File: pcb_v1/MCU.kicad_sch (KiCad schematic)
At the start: 3 parts, among them U4 ESP32-S3-MINI-1, U6 STM32F103RETx

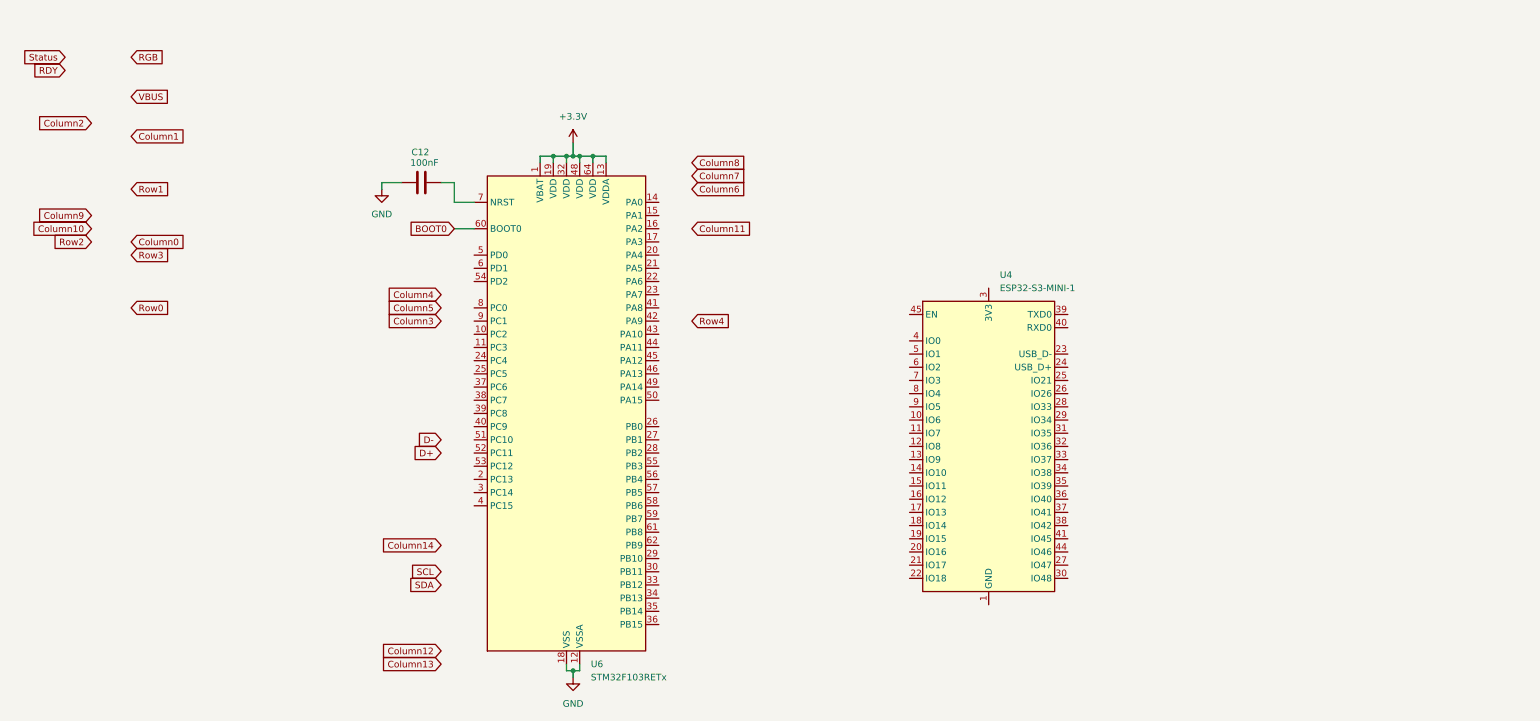
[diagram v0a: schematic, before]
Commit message: Updated wiring
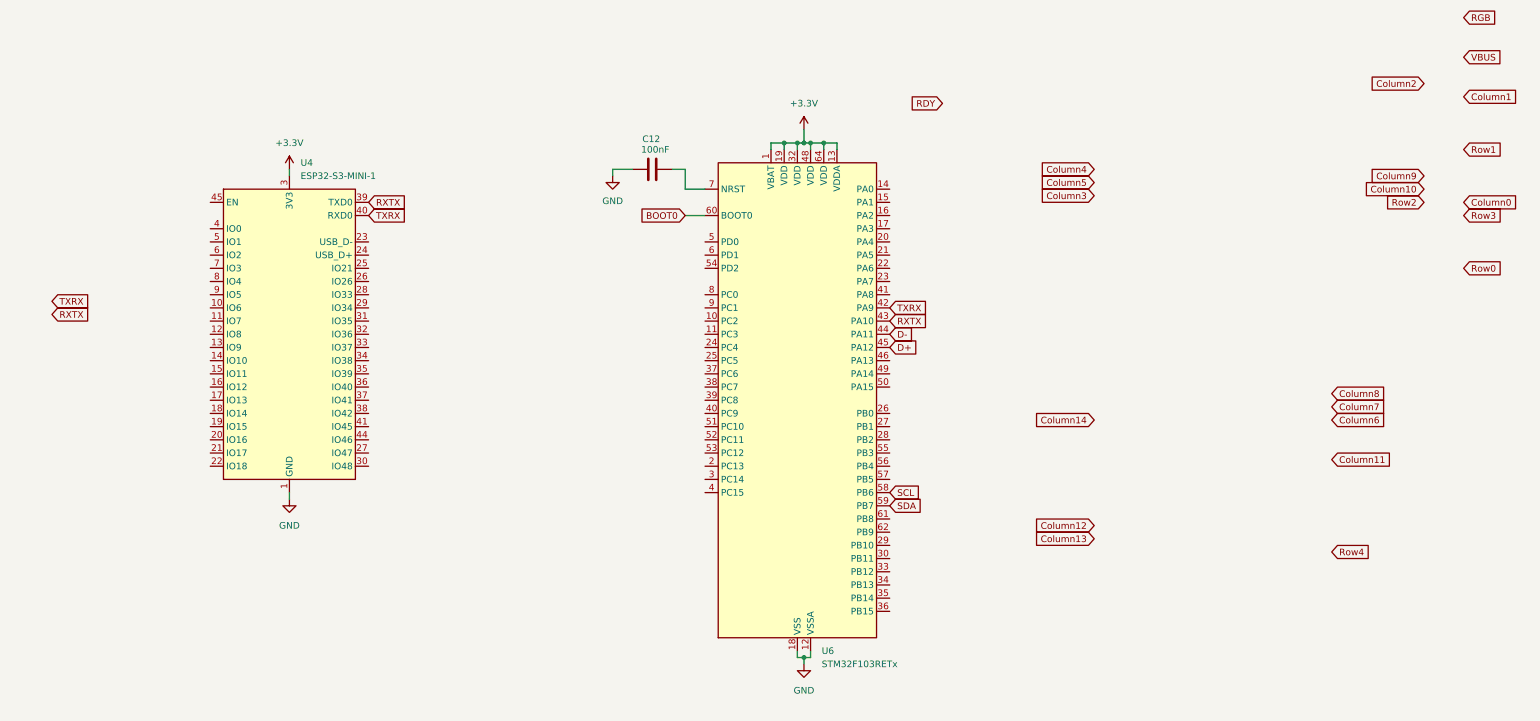
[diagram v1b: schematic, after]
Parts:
- C12: footprint Capacitor_SMD:C_0805_2012Metric -> Murata Capacitor:CAPC1608X90N
- U4: footprint RF_Module:ESP32-S2-MINI-1 -> ESP32-S3-MINI-1-N8:XCVR_ESP32-S3-MINI-1-N8
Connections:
- net +3.3V: now also U4.3 (3V3)
- net D+: now also U6.45 (PA12)
- net D-: now also U6.44 (PA11)
- net GND: now also U4.1 (GND), U4.2 (GND), U4.42 (GND), U4.43 (GND), U4.46 (GND), U4.47 (GND), U4.48 (GND), U4.49 (GND), U4.50 (GND), U4.51 (GND), U4.52 (GND), U4.53 (GND), U4.54 (GND), U4.55 (GND), U4.56 (GND), U4.57 (GND), U4.58 (GND), U4.59 (GND), U4.60 (GND), U4.61 (GND), U4.62 (GND), U4.63 (GND), U4.64 (GND), U4.65 (GND)
- net SCL: now also U6.58 (PB6)
- net SDA: now also U6.59 (PB7)
- net TXRX: now reaches U6.42 (PA9)
- net TXRX: now also U4.40 (RXD0)
- net RXTX: now reaches U6.43 (PA10)
- net RXTX: now also U4.39 (TXD0)
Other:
- moved on the sheet: C12, U4, U6

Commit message: Update Wiring
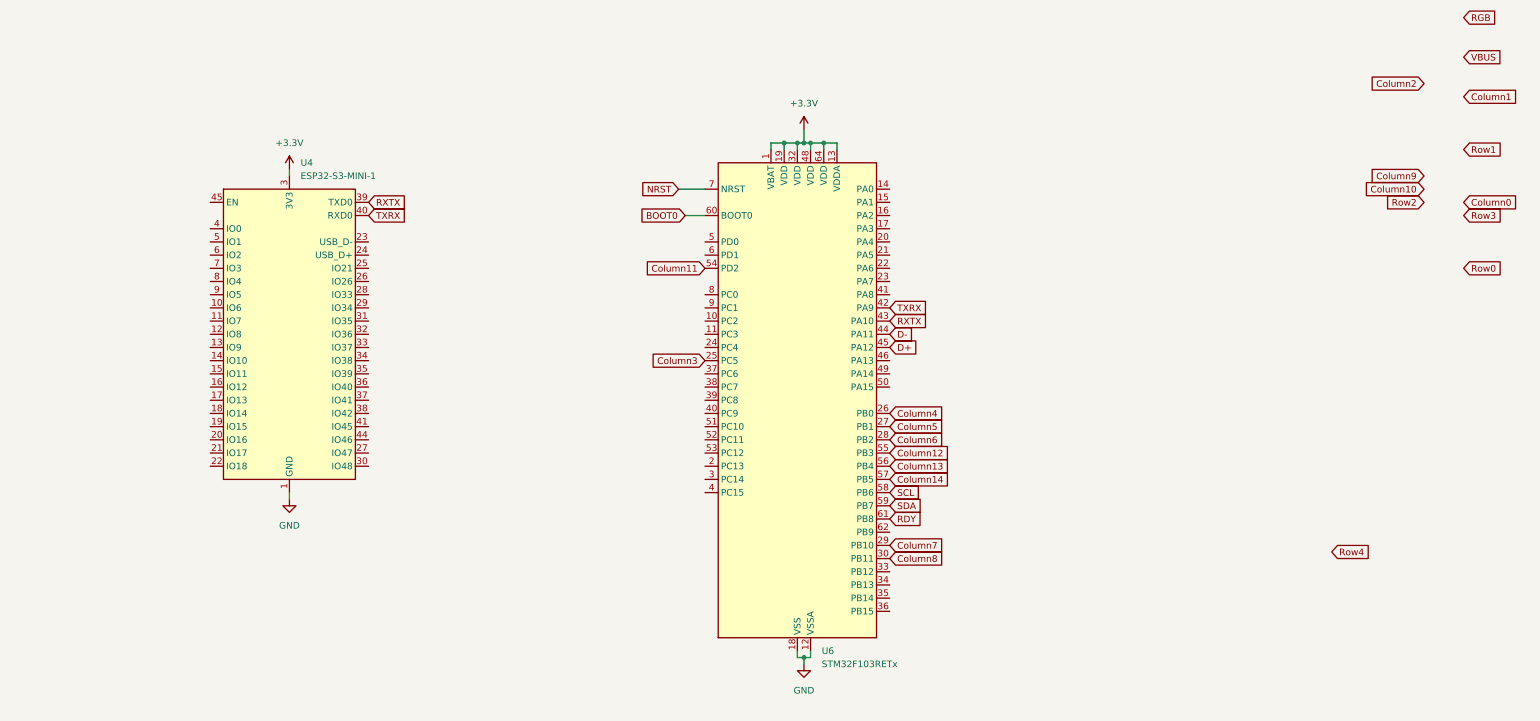
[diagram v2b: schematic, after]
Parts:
- removed C12: 100nF, Murata Capacitor:CAPC1608X90N, symbol Device:C
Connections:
- net Column11: now also U6.54 (PD2)
- net Column12: now also U6.55 (PB3)
- net Column13: now also U6.56 (PB4)
- net Column14: now also U6.57 (PB5)
- net Column3: now also U6.25 (PC5)
- net Column4: now also U6.26 (PB0)
- net Column5: now also U6.27 (PB1)
- net Column6: now also U6.28 (PB2)
- net Column7: now also U6.29 (PB10)
- net Column8: now also U6.30 (PB11)
- net RDY: now also U6.61 (PB8)
- net NRST: now reaches U6.7 (NRST)
